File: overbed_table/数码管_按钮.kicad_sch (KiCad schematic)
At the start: 1 part, among them U3 TM1638

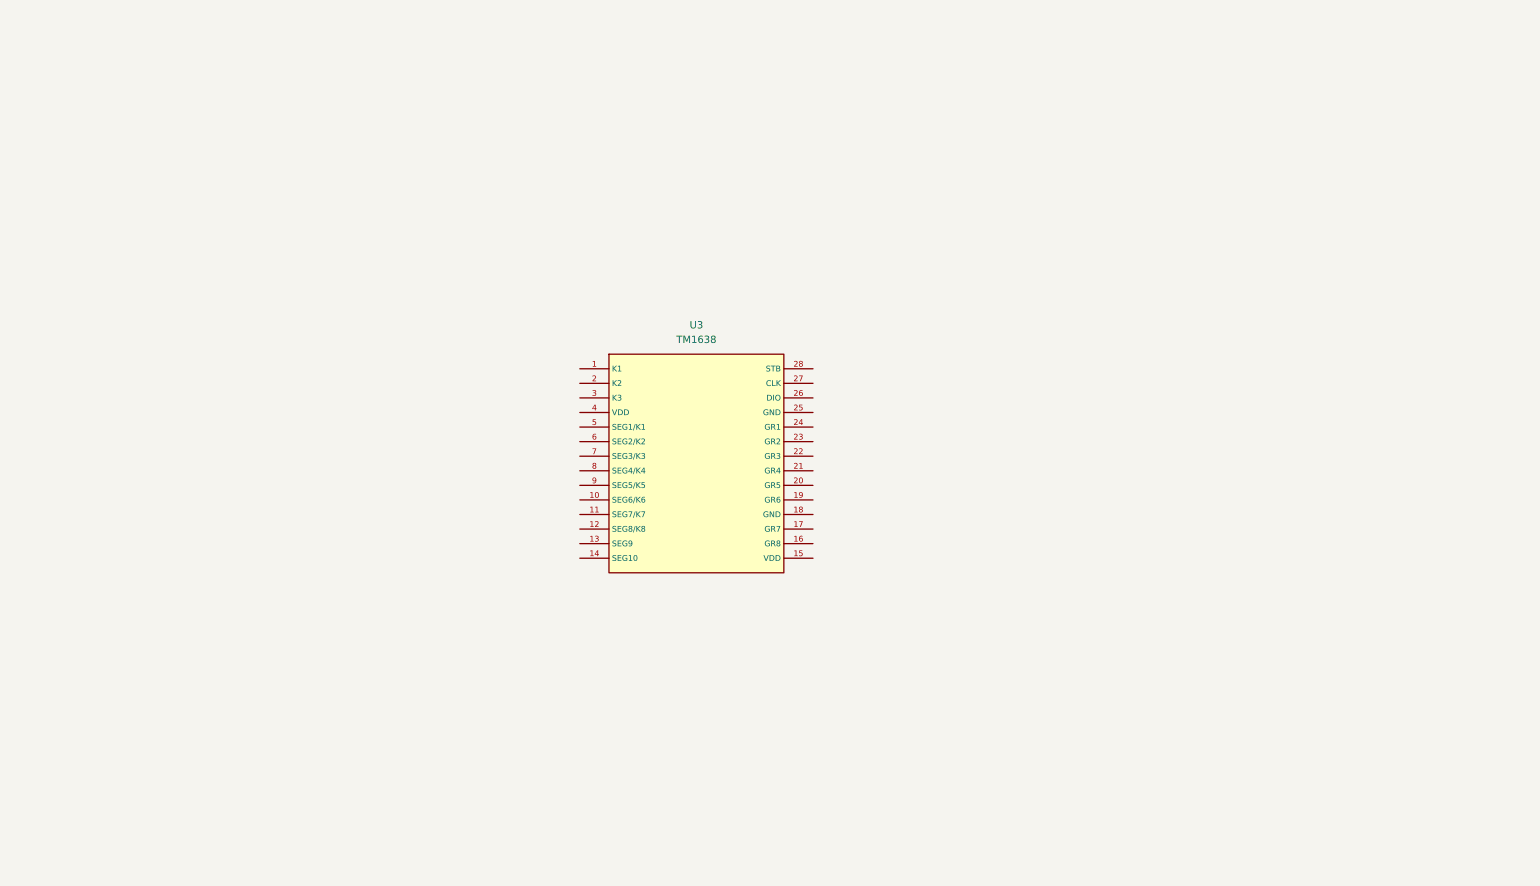
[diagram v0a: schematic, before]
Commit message: 更新驱动
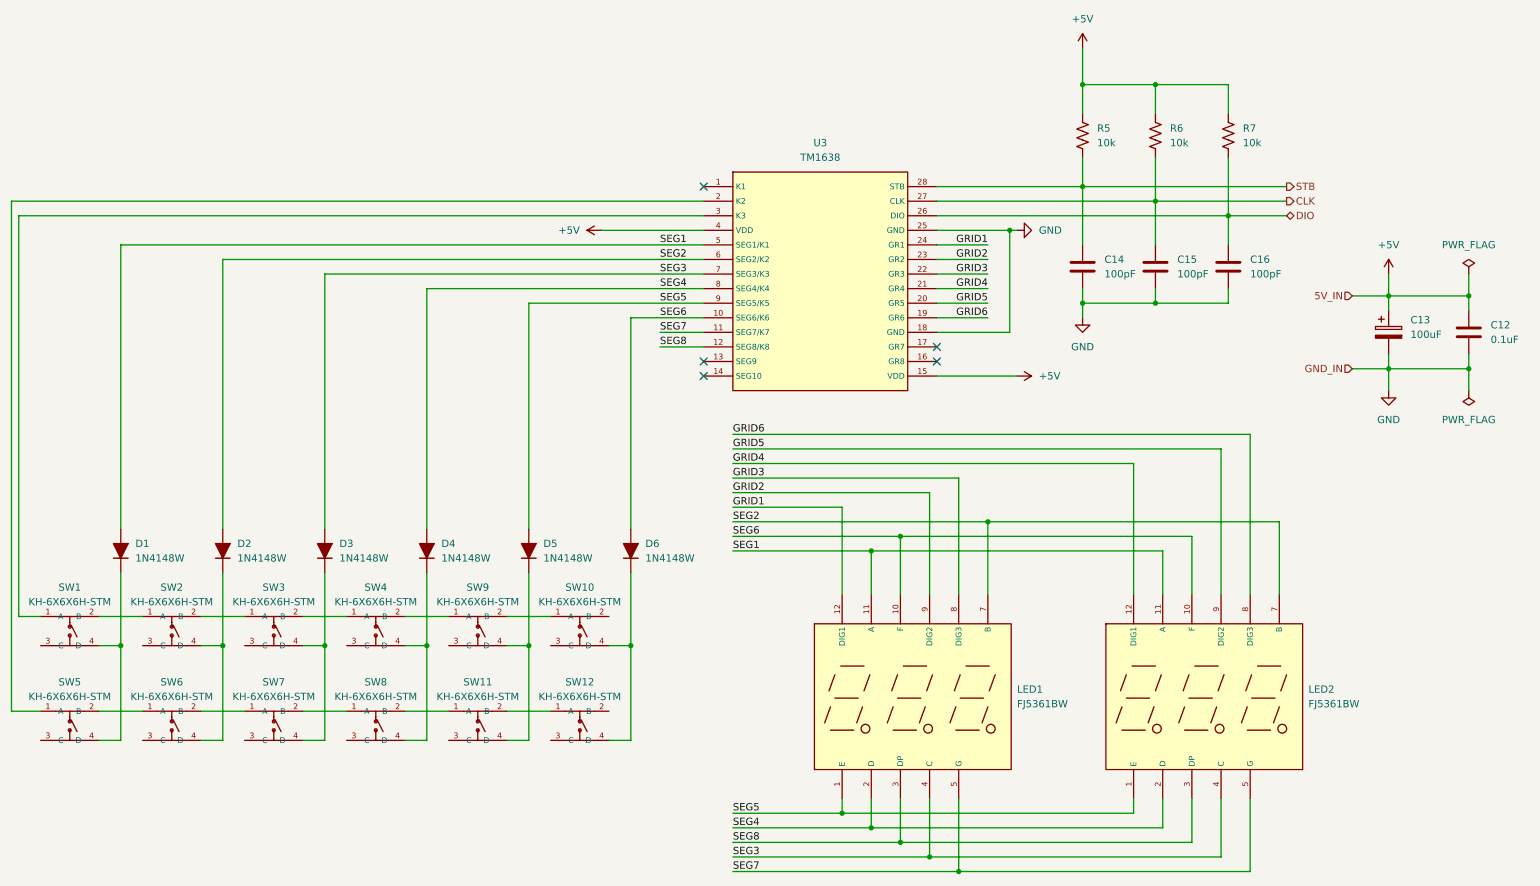
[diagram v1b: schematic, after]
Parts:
- added C12: 0.1uF, Button_Switch_SMD:Nidec_Copal_CAS-120A, symbol Device:C
- added C13: 100uF, Button_Switch_SMD:Nidec_Copal_CAS-120A, symbol Device:C_Polarized
- added C14, C15, C16: 100pF, Button_Switch_SMD:Nidec_Copal_CAS-120A, symbol Device:C
- added D1, D2, D3, D4, D5, D6: 1N4148W, PCM_Diode_SMD_AKL:D_SOD-123, symbol PCM_Diode_AKL:1N4148W
- added LED1, LED2: FJ5361BW, lcsc_footprints:C2938342_LED-SEG-TH_11P-L37_5-W19_0-P2_54-LS15_2-BL, symbol lcsc_imported:FJ5361BW
- added R5, R6, R7: 10k, PCM_SparkFun-Resistor:R_0603_1608Metric, symbol PCM_SparkFun-Resistor:R
- added SW1, SW10, SW11, SW12, SW2, SW3, SW4, SW5, SW6, SW7, SW8, SW9: KH-6X6X6H-STM, lcsc_footprints:C2837532_SW-SMD_4P-L6_0-W6_0-P4_50-LS9_0_KH-6X6X6H-STM, symbol lcsc_imported:KH-6X6X6H-STM
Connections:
- net SEG6: now reaches U3.10 (SEG6/K6)
- net SEG6: now also D6.2 (A), LED1.10 (F), LED2.10 (F)
- net SEG7: now reaches U3.11 (SEG7/K7)
- net SEG7: now also LED1.5 (G), LED2.5 (G)
- net SEG8: now reaches U3.12 (SEG8/K8)
- net SEG8: now also LED1.3 (DP), LED2.3 (DP)
- net +5V: now reaches U3.15 (VDD)
- net +5V: now also U3.4 (VDD), C12.1, C13.1, R5.2, R6.2, R7.2
- net GND: now reaches U3.18 (GND)
- net GND: now also U3.25 (GND), C12.2, C13.2, C14.2, C15.2, C16.2
- net GRID6: now reaches U3.19 (GR6)
- net GRID6: now also LED2.8 (DIG3)
- net at U3.2 (K2): now also SW5.1 (A)
- net GRID5: now reaches U3.20 (GR5)
- net GRID5: now also LED2.9 (DIG2)
- net GRID4: now reaches U3.21 (GR4)
- net GRID4: now also LED2.12 (DIG1)
- net GRID3: now reaches U3.22 (GR3)
- net GRID3: now also LED1.8 (DIG3)
- net GRID2: now reaches U3.23 (GR2)
- net GRID2: now also LED1.9 (DIG2)
- net GRID1: now reaches U3.24 (GR1)
- net GRID1: now also LED1.12 (DIG1)
- net DIO: now reaches U3.26 (DIO)
- net DIO: now also C16.1, R7.1
- net CLK: now reaches U3.27 (CLK)
- net CLK: now also C15.1, R6.1
- net STB: now reaches U3.28 (STB)
- net STB: now also C14.1, R5.1
- net at U3.3 (K3): now also SW1.1 (A)
- net SEG1: now reaches U3.5 (SEG1/K1)
- net SEG1: now also D1.2 (A), LED1.11 (A), LED2.11 (A)
- net SEG2: now reaches U3.6 (SEG2/K2)
- net SEG2: now also D2.2 (A), LED1.7 (B), LED2.7 (B)
- net SEG3: now reaches U3.7 (SEG3/K3)
- net SEG3: now also D3.2 (A), LED1.4 (C), LED2.4 (C)
- net SEG4: now reaches U3.8 (SEG4/K4)
- net SEG4: now also D4.2 (A), LED1.2 (D), LED2.2 (D)
- net SEG5: now reaches U3.9 (SEG5/K5)
- net SEG5: now also D5.2 (A), LED1.1 (E), LED2.1 (E)
- new net: SW5.2 (B), SW6.1 (A)
- new net: SW6.2 (B), SW7.1 (A)
- new net: D2.1 (K), SW2.4 (D), SW6.4 (D)
- new net: D1.1 (K), SW1.4 (D), SW5.4 (D)
- new net: D6.1 (K), SW10.4 (D), SW12.4 (D)
- new net: D3.1 (K), SW3.4 (D), SW7.4 (D)
- new net: SW1.2 (B), SW2.1 (A)
- new net: SW11.1 (A), SW8.2 (B)
- new net: SW11.2 (B), SW12.1 (A)
- new net: D5.1 (K), SW11.4 (D), SW9.4 (D)
- new net: SW4.2 (B), SW9.1 (A)
- new net: SW10.1 (A), SW9.2 (B)
- new net: SW2.2 (B), SW3.1 (A)
- new net: SW3.2 (B), SW4.1 (A)
- new net: D4.1 (K), SW4.4 (D), SW8.4 (D)
- new net: SW7.2 (B), SW8.1 (A)
- no-connect marks 0 -> 5
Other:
- moved on the sheet: U3
